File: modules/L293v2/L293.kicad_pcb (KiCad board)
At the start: 2 copper layers, 40.6 x 40.6 mm, 43 parts, among them J1 2, J10 11, J11 12, J12 13, J13 A0, J14 A1, J15 A2, J16 A3, J17 A4, J18 A5, J19 Vcc, J2 3, J20 Gnd, J21 Pwr, J22 M1, J23 M2, J24 Conn_01x01_Male, J25 Conn_01x01_Male, J3 4, J4 5, J5 6, J6 7, J7 8, J8 9, J9 10, U1 74LS175, U5 L293D, U6 L4940

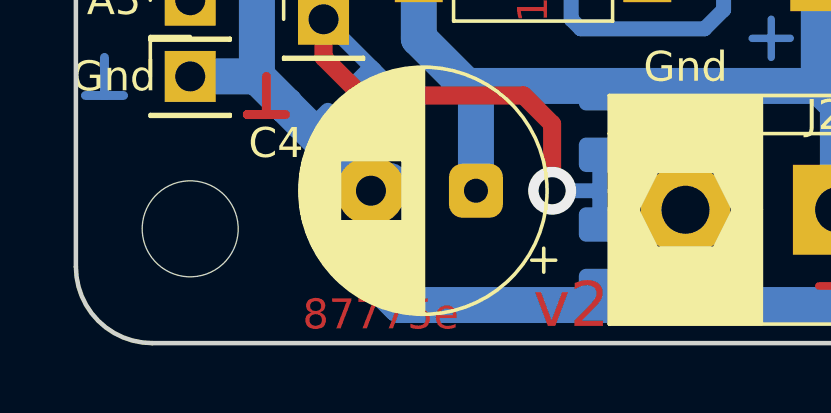
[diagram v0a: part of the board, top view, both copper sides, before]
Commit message: Fix hash, add gerber
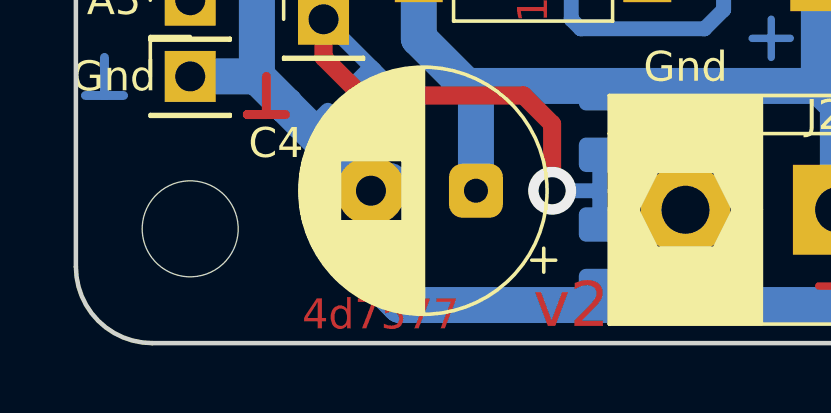
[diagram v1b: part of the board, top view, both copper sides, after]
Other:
- board text added: "4d7577"
- board text removed: "87775e"
